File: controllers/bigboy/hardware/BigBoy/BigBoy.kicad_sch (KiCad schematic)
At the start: 52 parts, among them J3 3.3V, J3 5V, J4 3.3V, J4 5V, J6 Conn_ST_STDC14, SW1 UB1/2, SW1 ~{RESET}, U29 STM32H743BITx, U3 AP7361EA-33E-13

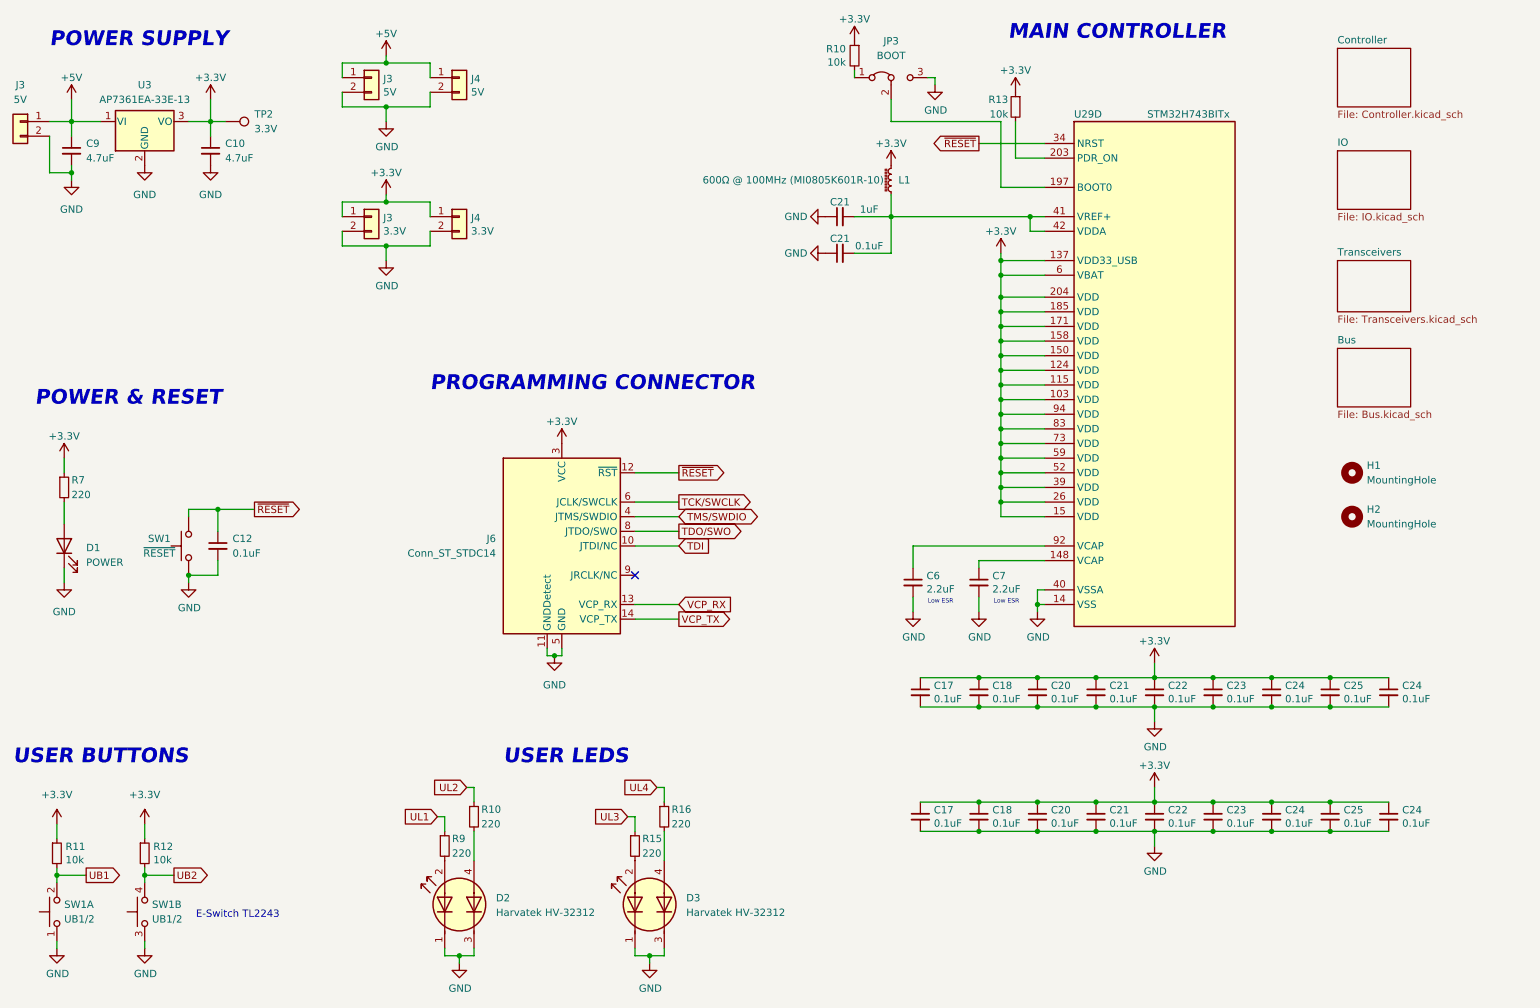
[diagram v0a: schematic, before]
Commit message: BigBoy Rev.1 is complete and ready to order
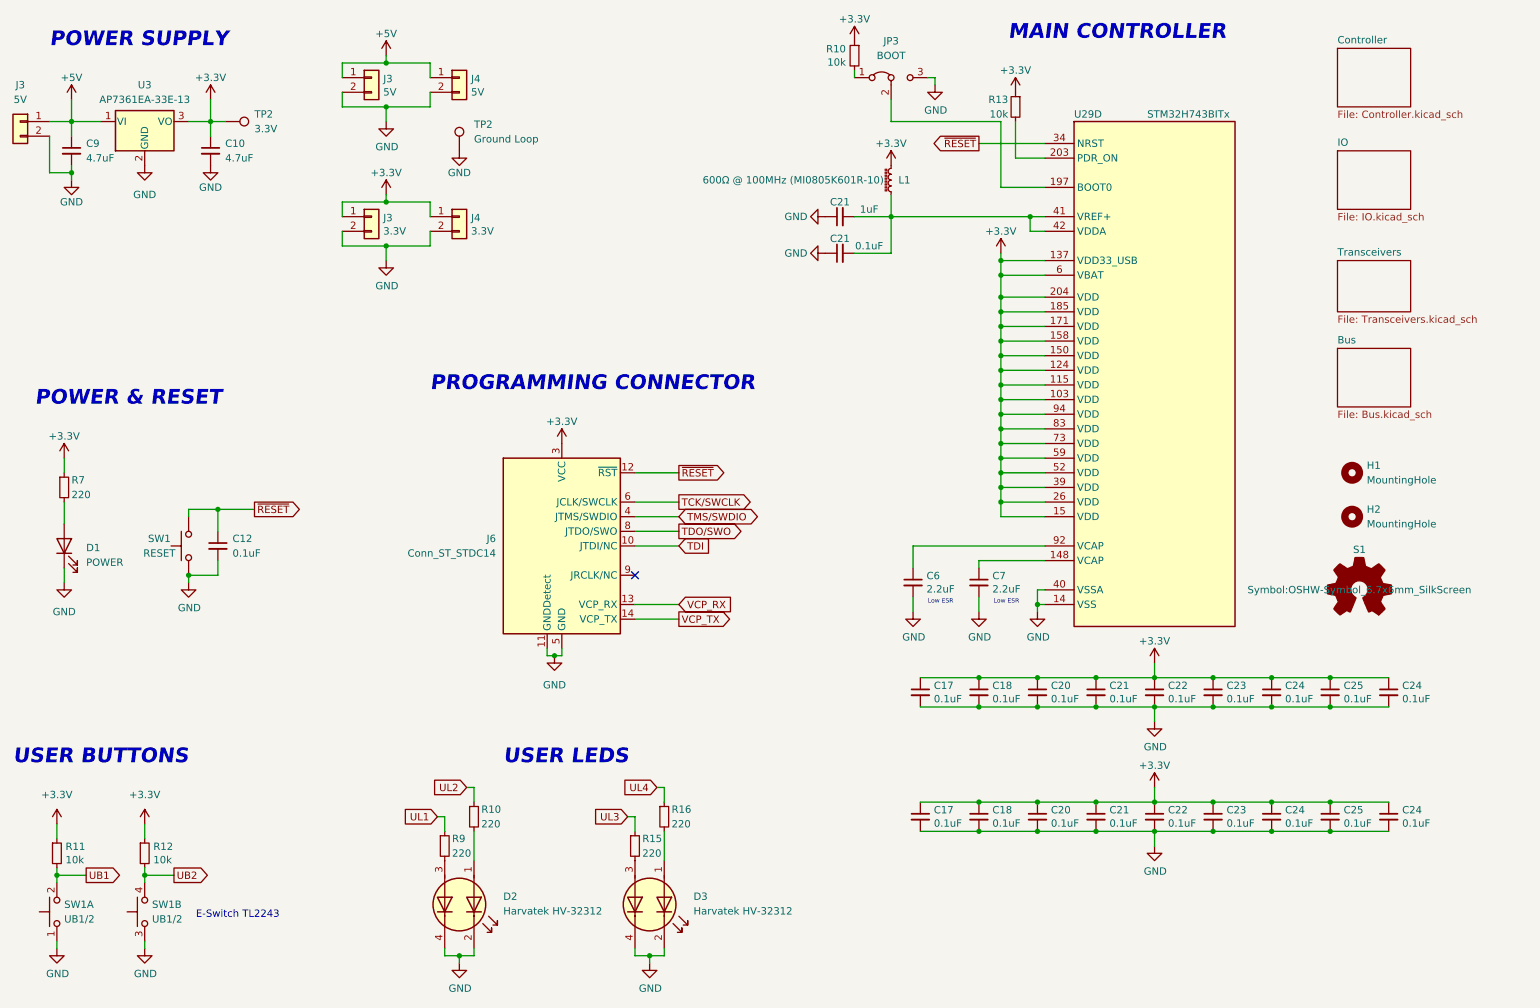
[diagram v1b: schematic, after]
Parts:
- added S1: Logo_Open_Hardware_Small, Symbol:OSHW-Symbol_6.7x6mm_SilkScreen, symbol Graphic:Logo_Open_Hardware_Small
- added TP2: Ground Loop, TestPoint:TestPoint_Loop_D2.60mm_Drill1.6mm_Beaded, symbol Connector:TestPoint
- D2, D3: footprint Computie_Miscellaneous:Dialight 553-0xxxF -> Computie_Miscellaneous:Harvatek_HV-32312-260-2SUB; symbol Device:LED_Dual_KAKA -> Device:LED_Dual_AKAK
- SW1: footprint Computie_Miscellaneous:E-Switch TL2243 -> Computie_Miscellaneous:E-Switch_TL2243
- SW1: value ~{RESET} -> RESET
- U29: footprint Computie_SMT:LQFP-208_28x28mm_P0.5mm -> Package_QFP:LQFP-208_28x28mm_P0.5mm
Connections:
- net GND: now also D2.2 (K1), D2.4 (K2), D3.2 (K1), D3.4 (K2), TP2.1; no longer D2.1 (A1), D2.3 (A2), D3.1 (A1), D3.3 (A2)
- net at R15.2: now also D3.3 (A2); no longer D3.2 (K1)
- net at R9.2: now also D2.3 (A2); no longer D2.2 (K1)
- net at R10.2: now also D2.1 (A1); no longer D2.4 (K2)
- net at R16.2: now also D3.1 (A1); no longer D3.4 (K2)
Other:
- moved on the sheet: D2, D3
